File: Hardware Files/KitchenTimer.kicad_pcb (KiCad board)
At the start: 2 copper layers, 100 x 100 mm, 81 parts, among them J1 Conn_01x04, J2 USB_B_Micro, J3 Battery, Q14 -30V 12A 14mΩ @ 8A, Q15 20V 7.5A 24mΩ @ 2.5Vgs, Q16 P 1V 250uA 4A SOT-23, Q17 P 1V 250uA 4A SOT-23, Q18 P 1V 250uA 4A SOT-23, Q19 P 1V 250uA 4A SOT-23, Q20 P 1V 250uA 4A SOT-23, SW1 SW_SPST, SW2 SW_SPST, SW3 SW_Push_Dual, SW4 SW_Push_Dual, SW5 SW_Push_Dual, SW6 SW_Push_Dual, U11 74HC595, U3 ESP-WROOM-02D, U4 AP34063S8G-13, U5 TP4056, U6 AP9101CK6, U7 NCP1117ST50T3G, U8 NCP1117ST33T3G, U9 74HC595

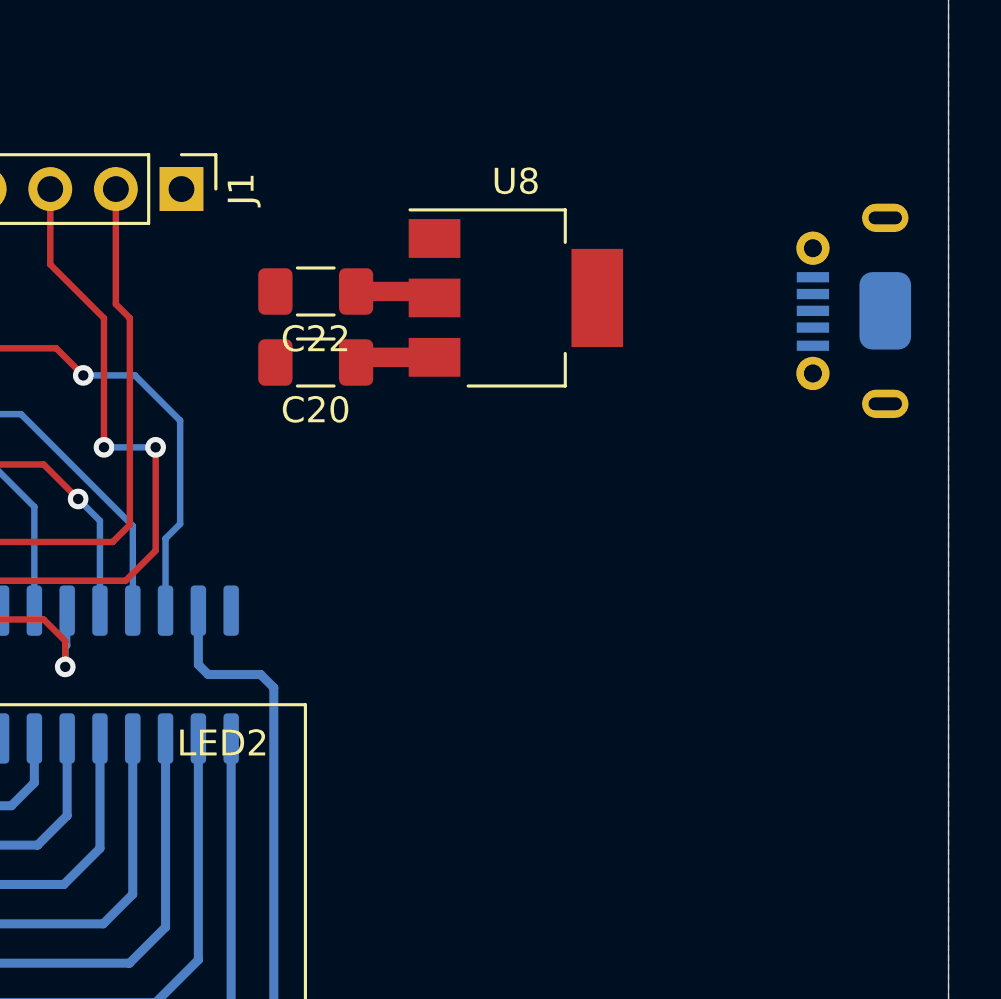
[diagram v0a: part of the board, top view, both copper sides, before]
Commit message: update layout
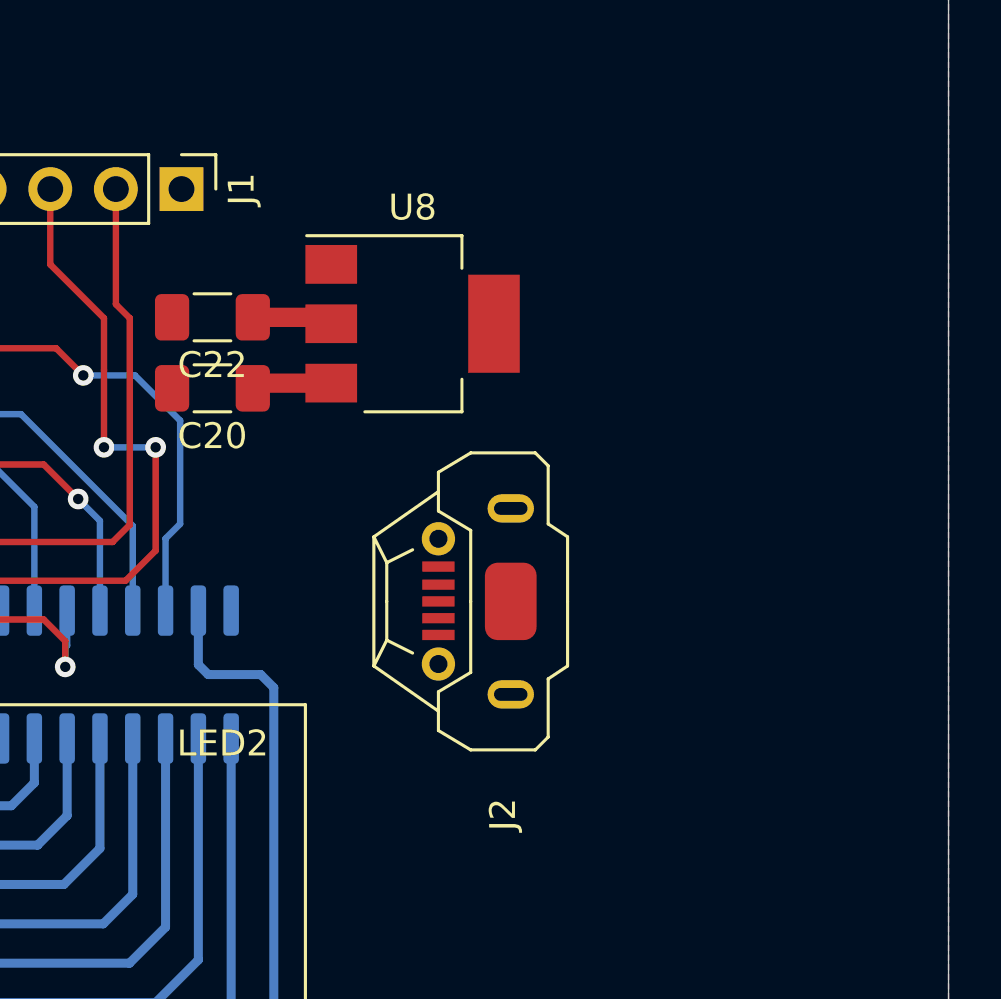
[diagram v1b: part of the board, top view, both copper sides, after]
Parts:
- J2: moved to F.Cu
- moved J2 18.4 mm to (327.0, -217.5), turned to 270 degrees
- moved C20 4.12 mm to (318.2, -225.8)
- moved C22 4.12 mm to (318.2, -228.5)
- moved U8 4.12 mm to (326.0, -228.2)
